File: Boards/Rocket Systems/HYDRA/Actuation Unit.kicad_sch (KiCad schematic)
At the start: 37 parts, among them K1 G3VM-31DR_TR05_, Q6 2N7002H6327XTSA2, Q7 2N7002H6327XTSA2, U17 DRV103H, U18 DRV103H, U19 DRV103H, U20 DRV103H, U21 NCR321UX, U22 SQJA36EP-T1_GE3, U23 SQJA36EP-T1_GE3, U24 SQJA36EP-T1_GE3

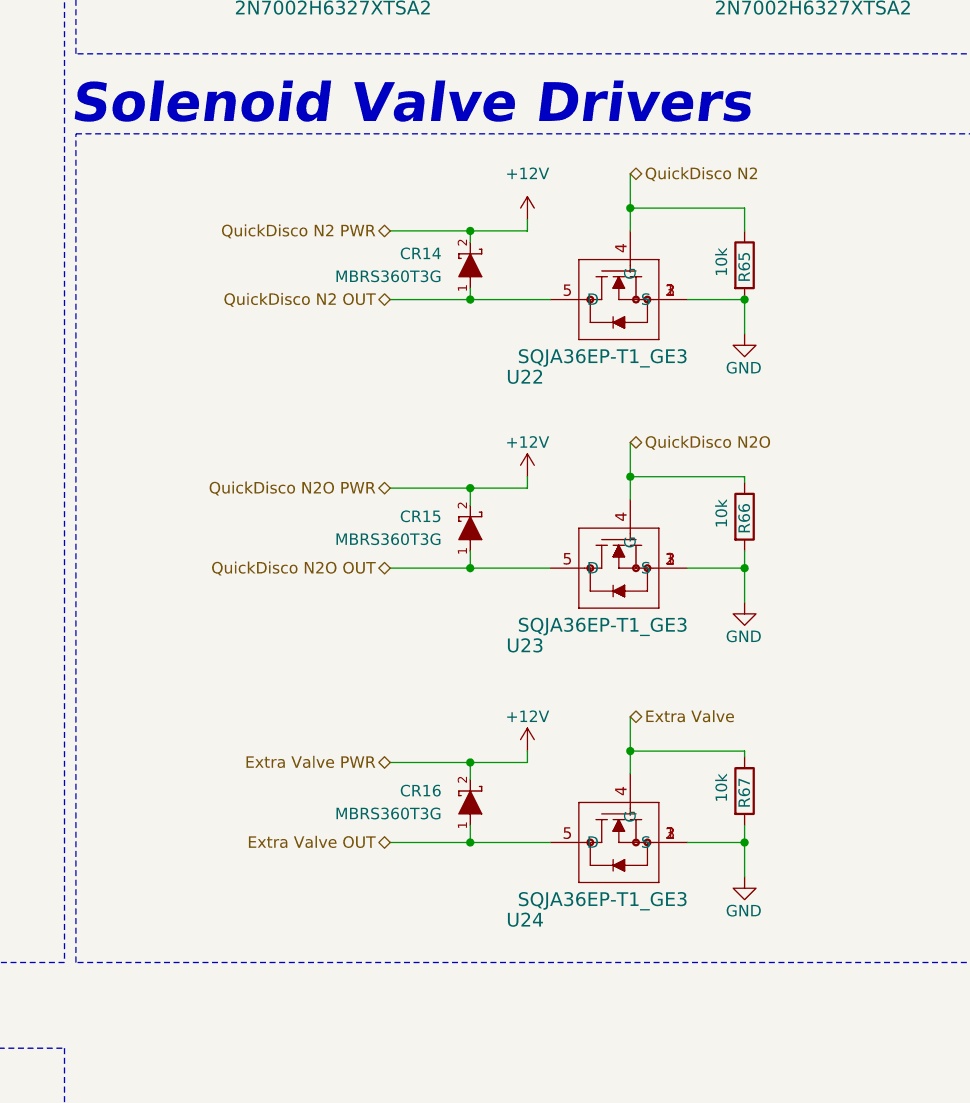
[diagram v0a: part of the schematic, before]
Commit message: DFM checks, Avionics Updates
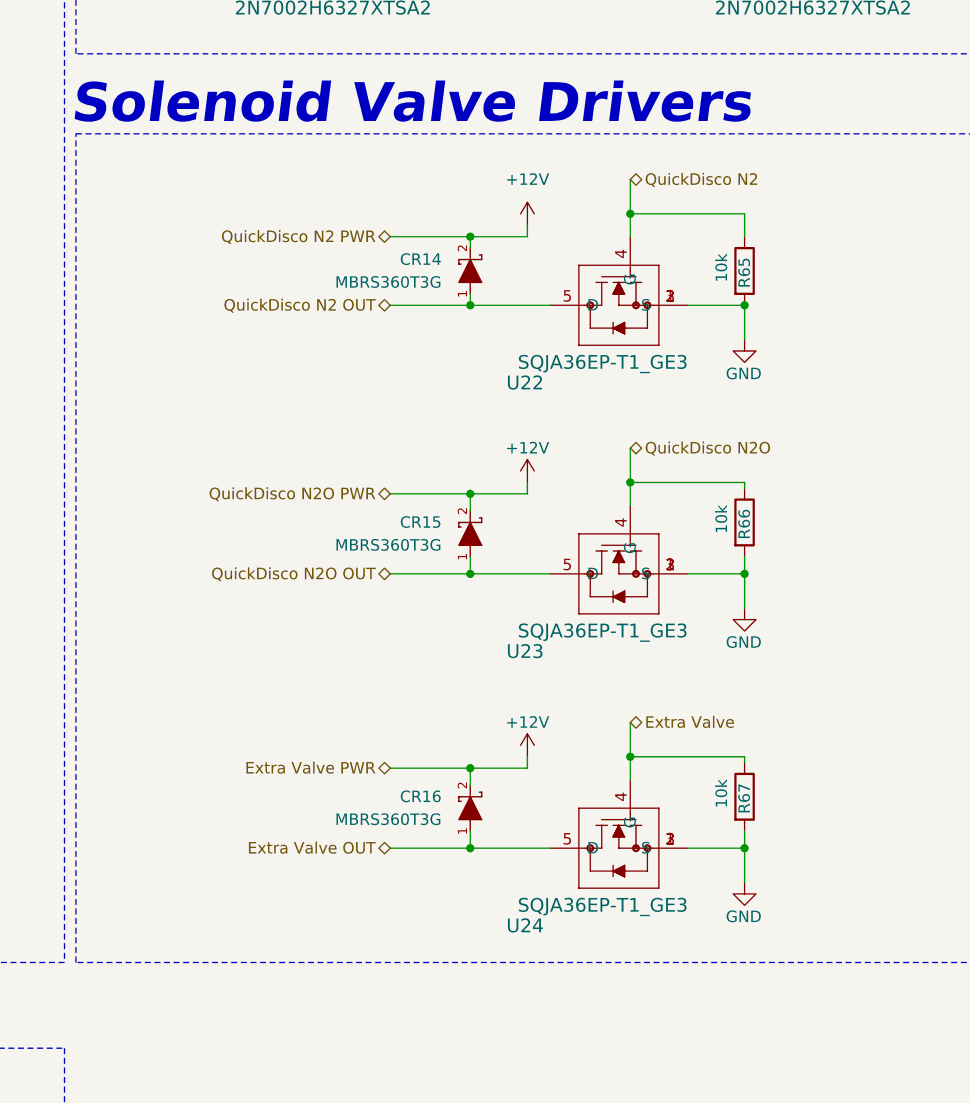
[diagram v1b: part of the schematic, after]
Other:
- moved on the sheet: CR14, CR15, CR16, R65, R66, R67, U22, U23, U24

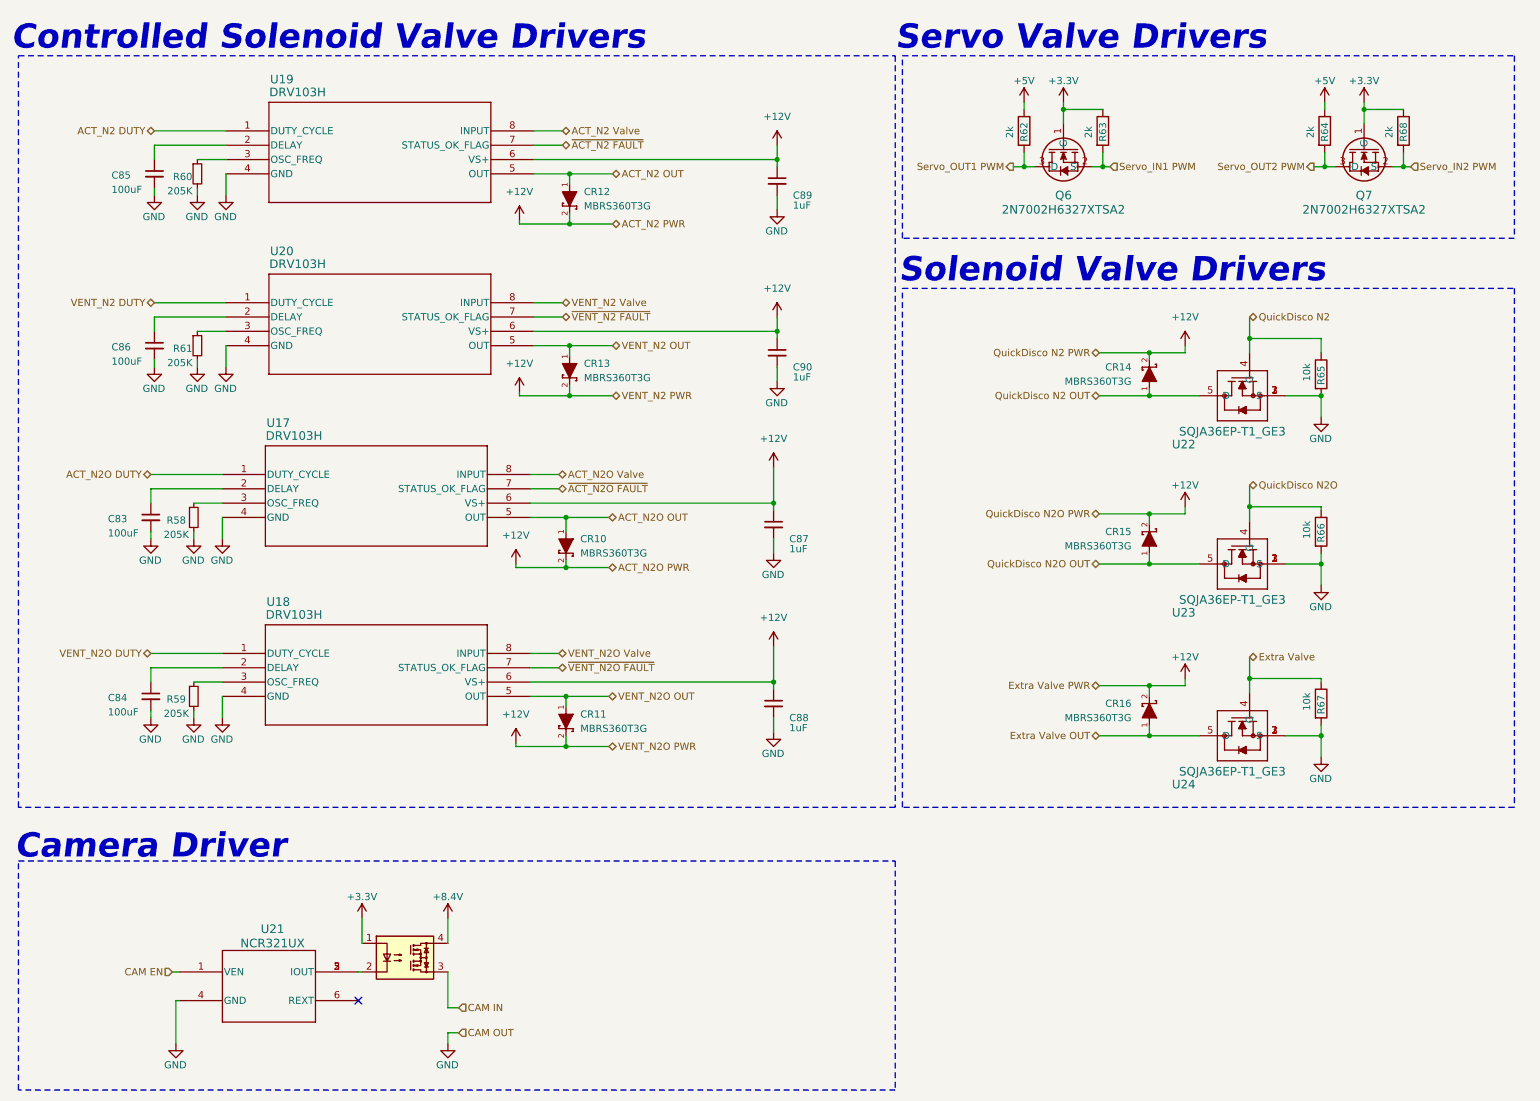
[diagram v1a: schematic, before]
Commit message: Elytra Update and HYDRA Update
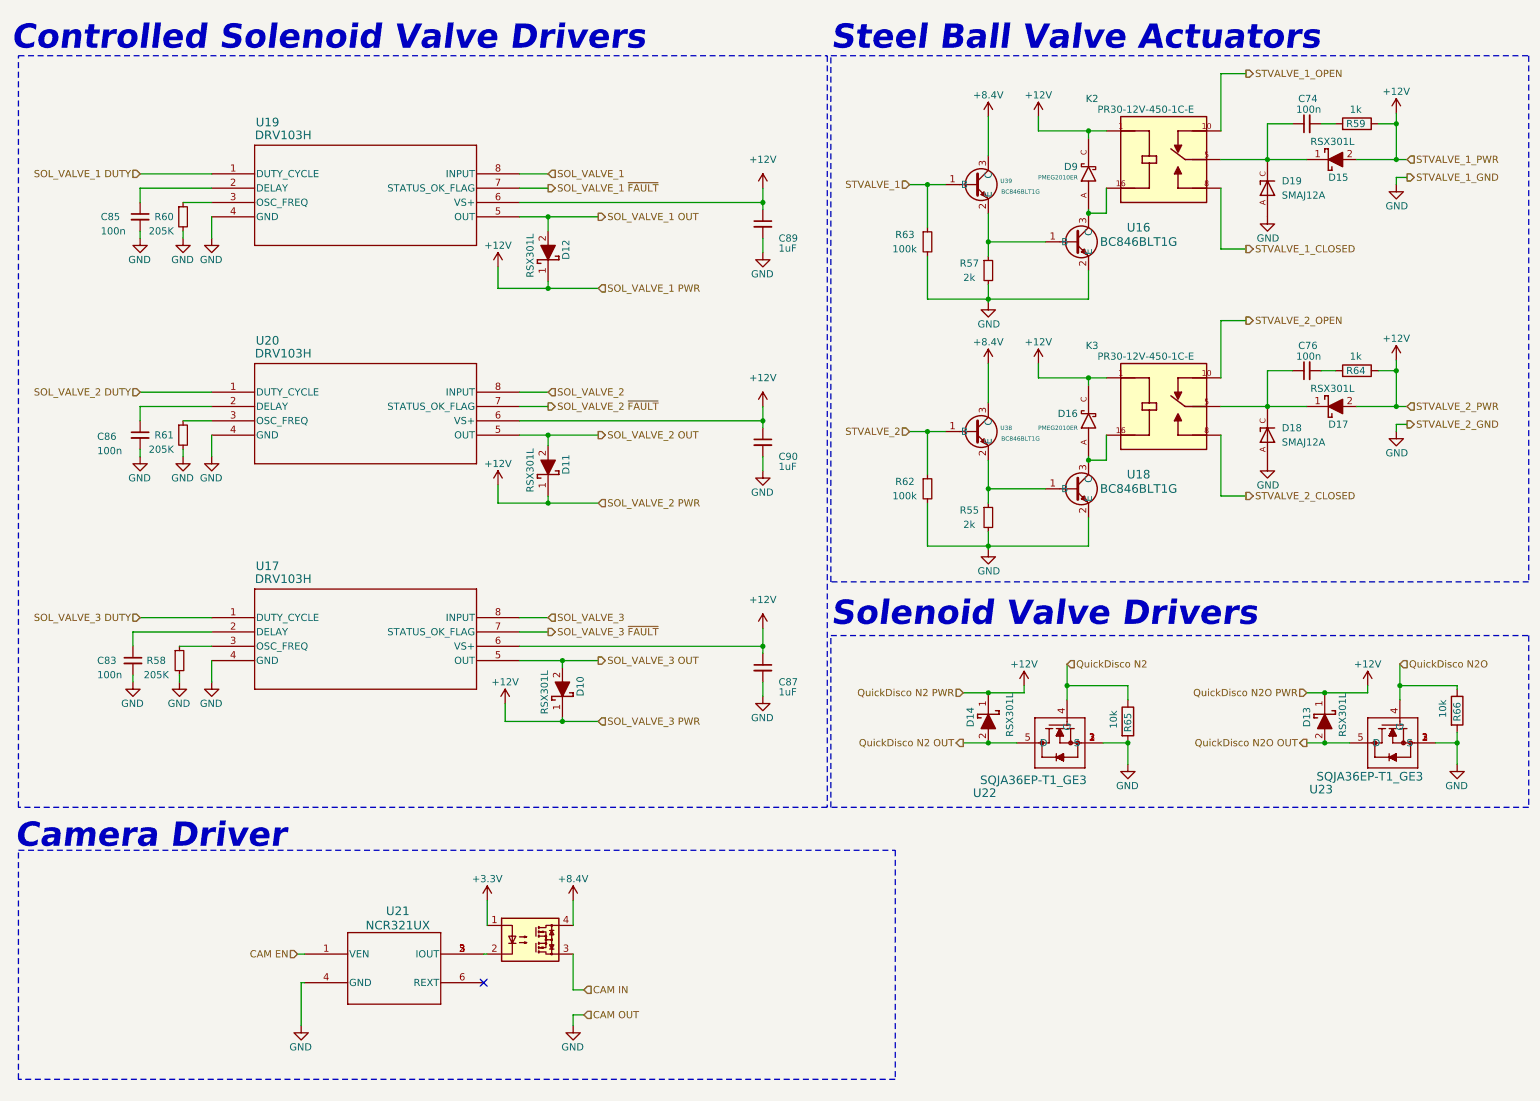
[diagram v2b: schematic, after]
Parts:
- removed C84: 100uF, symbol Device:C_Small
- removed C88: 1uF, symbol Device:C_Small
- removed CR10, CR11, CR12, CR13, CR14, CR15, CR16: MBRS360T3G, MBRS360T3G:DIODE_SMC_7P15X6P25_ONS-M, symbol MBRS360T3G:MBRS360T3G
- removed Q6, Q7: 2N7002H6327XTSA2, NMOS_2N7002:PG-SOT23-3-5_INF_MIN, symbol NMOS_2N7002:2N7002H6327XTSA2
- removed R59: 205K, symbol Device:R_Small
- removed R62, R63, R68: 2k, Resistor-0402:RES_0402, symbol Device:R
- removed R67: 10k, Resistor-0402:RES_0402, symbol Device:R
- removed U18: DRV103H, DDA8, symbol DRV103H:DRV103H
- removed U24: SQJA36EP-T1_GE3, PowerPAK_SO-8L_3_VIS, symbol SQJA36EP-T1-GE3:SQJA36EP-T1_GE3
- added C74, C76: 100n, Capacitor-0603:Capacitor_0603, symbol Device:C_Small
- added D10, D11, D12, D13, D14, D15, D17: RSX301L, Diode-Schottky_RSX301L:DIOM5026X220N, symbol RSX301L-30DDTE25:RSX301L-30DDTE25
- added D16, D9: PMEG2010ER, Diode-Schottky_PMEG2010ER:SODFL3517X110N, symbol PMEG2010ER:PMEG2010ER
- added D18, D19: SMAJ12A, SMAJ12A:DIOM4325X250N, symbol SMAJ12A:SMAJ12A
- added K2, K3: PR30-12V-450-1C-E, PR30-12V-450-1C-E:RELAY_PR30-12V-450-1C-E, symbol PR30-12V-450-1C-E:PR30-12V-450-1C-E
- added R55, R57: 2k, Resistor-0603:RES_0603, symbol Device:R_Small
- added R59: 1k, Resistor-0805:RES_0805, symbol Device:R
- added R62, R63: 100k, Resistor-0603:RES_0603, symbol Device:R_Small
- added U16, U18, U38, U39: BC846BLT1G, BC846BLT1G:SOT-23_ONS, symbol BC846BLT1G:BC846BLT1G
- C83, C85, C86: value 100uF -> 100n; footprint (none) -> Capacitor-0603:Capacitor_0603
- R58, R60, R61: footprint (none) -> Resistor-0603:RES_0603
- R64: value 2k -> 1k; footprint Resistor-0402:RES_0402 -> Resistor-0805:RES_0805
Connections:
- net +5V is gone; now on net +12V: R64.1
- net +12V: now also D10.1 (K), D11.1 (K), D12.1 (K), D13.1 (K), D14.1 (K), D15.2 (A), D16.C, D17.2 (A), D9.C, K2.1, K3.1, R59.1
- net +8.4V: now also U38.3 (C), U39.3 (C)
- net GND: now also D18.A, D19.A, R55.2, R57.2, R62.2, R63.2, U16.2 (E), U18.2 (E)
- net QuickDisco N2 OUT: now also D14.2 (A)
- net QuickDisco N2O OUT: now also D13.2 (A)
- net ACT_N2 DUTY renamed SOL_VALVE_1 DUTY
- net ACT_N2 OUT renamed SOL_VALVE_1 OUT
- net SOL_VALVE_1 OUT: now also D12.2 (A)
- net ACT_N2 Valve renamed SOL_VALVE_1
- net ACT_N2O DUTY renamed SOL_VALVE_3 DUTY
- net ACT_N2O OUT renamed SOL_VALVE_3 OUT
- net SOL_VALVE_3 OUT: now also D10.2 (A)
- net ACT_N2O Valve renamed SOL_VALVE_3
- net Servo_OUT2 PWM: no longer names the net of R64.2
- net Servo_OUT2 PWM: now also C76.2
- net VENT_N2 DUTY renamed SOL_VALVE_2 DUTY
- net VENT_N2 OUT renamed SOL_VALVE_2 OUT
- net SOL_VALVE_2 OUT: now also D11.2 (A)
- net VENT_N2 Valve renamed SOL_VALVE_2
- net ~{ACT_N2 FAULT} renamed SOL_VALVE_1 ~{FAULT}
- net ~{ACT_N2O FAULT} renamed SOL_VALVE_3 ~{FAULT}
- net ~{VENT_N2 FAULT} renamed SOL_VALVE_2 ~{FAULT}
- new net: C76.1, D17.1 (K), D18.C, K3.5
- new net: D16.A, K3.16, U18.3 (C)
- new net: D9.A, K2.16, U16.3 (C)
- new net: C74.1, D15.1 (K), D19.C, K2.5
- new net: R55.1, U18.1 (B), U38.2 (E)
- new net: R57.1, U16.1 (B), U39.2 (E)
- new net: C74.2, R59.2
- new net STVALVE_1: R63.1, U39.1 (B)
- new net STVALVE_1_CLOSED: K2.8
- new net STVALVE_1_OPEN: K2.10
- new net STVALVE_2: R62.1, U38.1 (B)
- new net STVALVE_2_CLOSED: K3.8
- new net STVALVE_2_OPEN: K3.10
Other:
- note added: "Steel Ball Valve Actuators"
- note removed: "Servo Valve Drivers"
- moved on the sheet: C83, C85, C86, C87, C89, C90, R58, R60, R61, R65, R66, U17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

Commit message: HYDRA Update - footprints and schematics
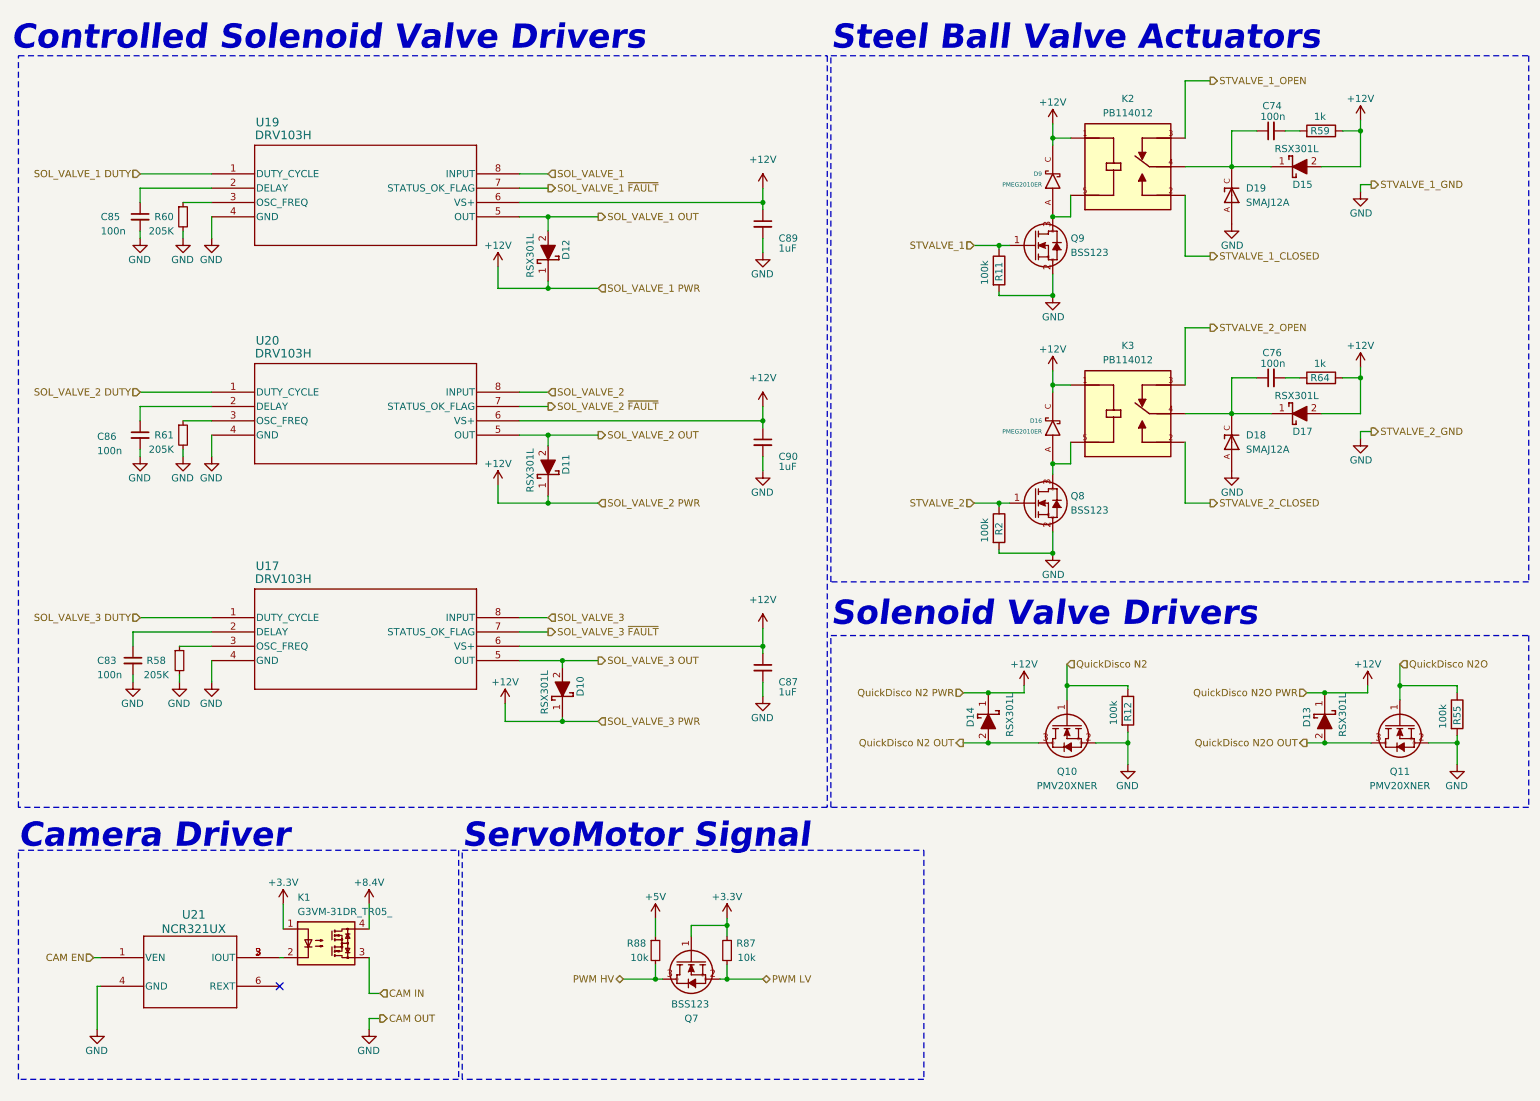
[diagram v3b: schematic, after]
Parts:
- removed K2, K3: PR30-12V-450-1C-E, PR30-12V-450-1C-E:RELAY_PR30-12V-450-1C-E, symbol PR30-12V-450-1C-E:PR30-12V-450-1C-E
- removed R55, R57: 2k, Resistor-0603:RES_0603, symbol Device:R_Small
- removed R62, R63: 100k, Resistor-0603:RES_0603, symbol Device:R_Small
- removed R65, R66: 10k, Resistor-0402:RES_0402, symbol Device:R
- removed U16, U18, U38, U39: BC846BLT1G, BC846BLT1G:SOT-23_ONS, symbol BC846BLT1G:BC846BLT1G
- removed U22, U23: SQJA36EP-T1_GE3, PowerPAK_SO-8L_3_VIS, symbol SQJA36EP-T1-GE3:SQJA36EP-T1_GE3
- added K2, K3: PB114012, PB134005, symbol PB114012:PB114012
- added Q10, Q11: PMV20XNER, SOT95P230X110-3N, symbol PMV20XNER:PMV20XNER
- added Q7, Q8, Q9: BSS123, SOT96P237X111-3N, symbol BSS123:BSS123
- added R11, R12, R2, R55: 100k, Resistor-0603:RES_0603, symbol Device:R
- added R87, R88: 10k, Resistor-0603:RES_0603, symbol Device:R_Small
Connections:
- net +12V: now also K2.1, K3.1
- net +3.3V: now also Q7.1 (G), R87.1
- net GND: now also Q10.2 (S), Q11.2 (S), Q8.2 (S), Q9.2 (S), R11.2, R12.2, R2.2, R55.2
- net QuickDisco N2: now also Q10.1 (G), R12.1
- net QuickDisco N2 OUT: now also Q10.3 (D)
- net QuickDisco N2O: now also Q11.1 (G), R55.1
- net QuickDisco N2O OUT: now also Q11.3 (D)
- net STVALVE_1: now also Q9.1 (G), R11.1
- net STVALVE_1_CLOSED: now also K2.2
- net STVALVE_1_OPEN: now also K2.3
- net STVALVE_2: now also Q8.1 (G), R2.1
- net STVALVE_2_CLOSED: now also K3.2
- net STVALVE_2_OPEN: now also K3.3
- net at C76.1, D17.1 (K), D18.C: now also K3.4
- net at D16.A: now also K3.5, Q8.3 (D)
- net at D9.A: now also K2.5, Q9.3 (D)
- net at C74.1, D15.1 (K), D19.C: now also K2.4
- new net +5V: R88.1
- new net PWM HV: Q7.3 (D), R88.2
- new net PWM LV: Q7.2 (S), R87.2
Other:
- note added: "ServoMotor Signal"
- moved on the sheet: C74, C76, D15, D16, D17, D18, D19, D9, R59, R64, U21
